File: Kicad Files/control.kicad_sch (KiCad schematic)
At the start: 77 parts, among them U35 74LS161, U36 SST39SF020, U37 SST39SF020, U38 SST39SF020, U39 SST39SF020

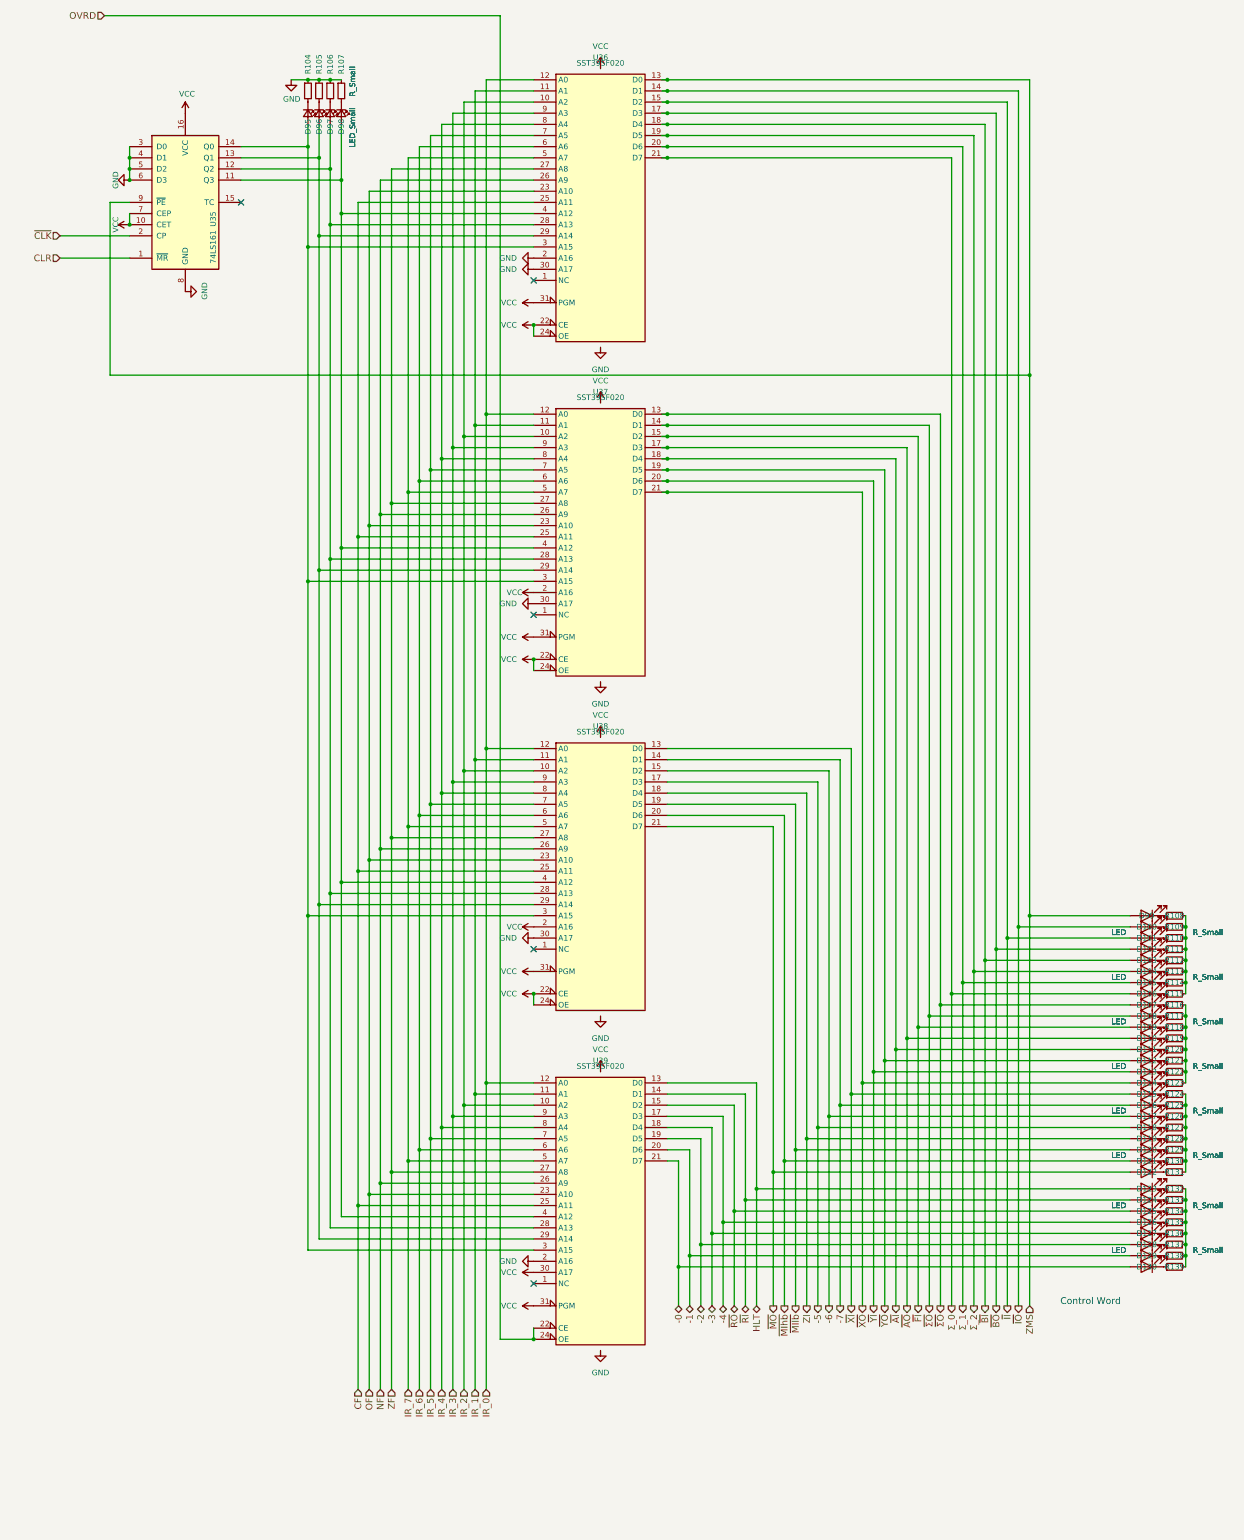
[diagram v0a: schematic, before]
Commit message: im sooo stupiiid
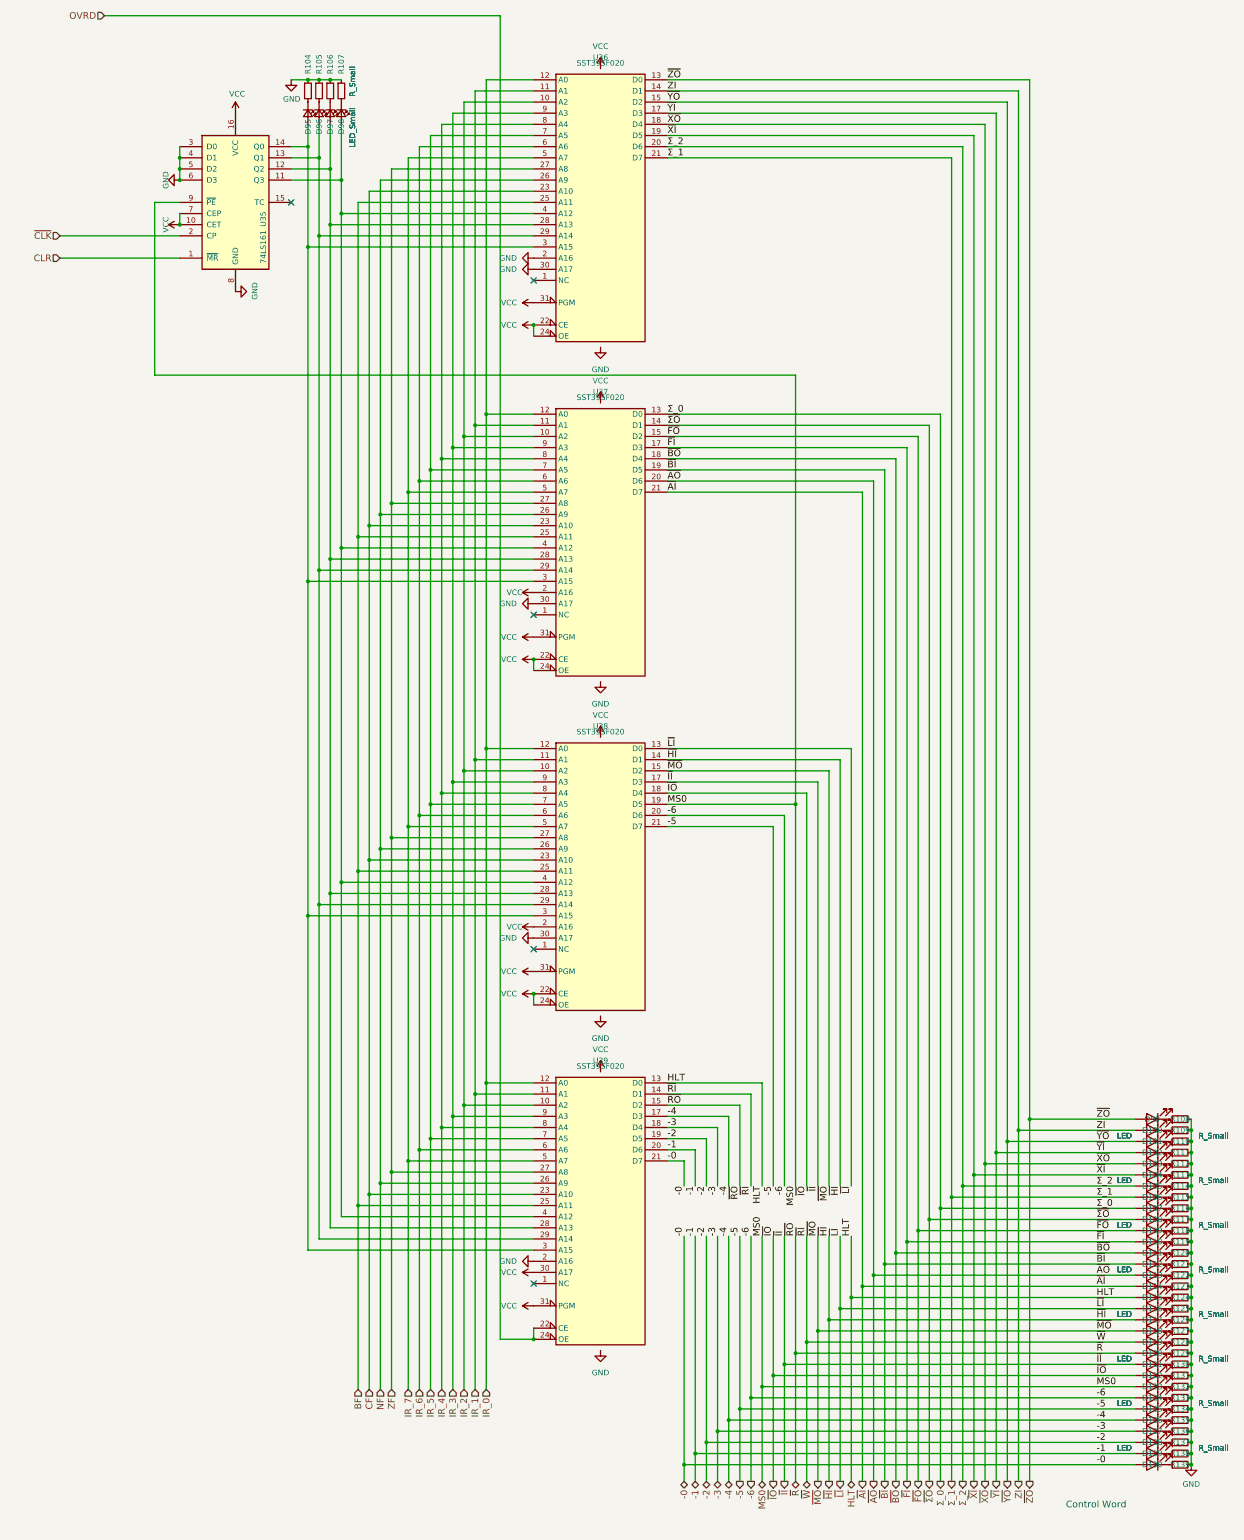
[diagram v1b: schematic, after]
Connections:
- net OF is gone; now on net CF: U36.23 (A10), U37.23 (A10), U38.23 (A10), U39.23 (A10)
- net -5: now also D125.2 (A), U38.21 (D7); no longer D118.2 (A), U38.17 (D3)
- net -6: now also D124.2 (A), U38.20 (D6); no longer D117.2 (A), U38.15 (D2)
- net CF: no longer U36.25 (A11), U37.25 (A11), U38.25 (A11), U39.25 (A11)
- net GND: now also R108.2, R109.2, R110.2, R111.2, R112.2, R113.2, R114.2, R115.2, R116.2, R117.2, R118.2, R119.2, R120.2, R121.2, R122.2, R123.2, R124.2, R125.2, R126.2, R127.2, R128.2, R129.2, R130.2, R131.2, R132.2, R133.2, R134.2, R135.2, R136.2, R137.2, R138.2, R139.2
- net HLT: now also D115.2 (A); no longer D123.2 (A)
- net ZI: now also D100.2 (A), U36.14 (D1); no longer D119.2 (A), U38.18 (D4)
- net ~{AI}: now also D114.2 (A), U37.21 (D7); no longer D111.2 (A), U37.18 (D4)
- net ~{AO}: now also D113.2 (A), U37.20 (D6); no longer D110.2 (A), U37.17 (D3)
- net ~{BI}: now also D112.2 (A), U37.19 (D5); no longer D103.2 (A), U36.18 (D4)
- net ~{BO}: now also D111.2 (A), U37.18 (D4); no longer D102.2 (A), U36.17 (D3)
- net ~{FI}: now also D110.2 (A), U37.17 (D3); no longer D109.2 (A), U37.15 (D2)
- net ~{II}: now also D121.2 (A), U38.17 (D3); no longer D101.2 (A), U36.15 (D2)
- net ~{IO}: now also D122.2 (A), U38.18 (D4); no longer D100.2 (A), U36.14 (D1)
- net ~{MO}: now also D118.2 (A), U38.15 (D2); no longer D122.2 (A), U38.21 (D7)
- net ~{XI}: now also D104.2 (A), U36.19 (D5); no longer D115.2 (A), U38.13 (D0)
- net ~{XO}: now also D103.2 (A), U36.18 (D4); no longer D114.2 (A), U37.21 (D7)
- net ~{YI}: now also D102.2 (A), U36.17 (D3); no longer D113.2 (A), U37.20 (D6)
- net ~{YO}: now also D101.2 (A), U36.15 (D2); no longer D112.2 (A), U37.19 (D5)
- net ~{ΣO}: no longer D107.2 (A), U37.13 (D0)
- net Σ_0: now also D107.2 (A), U37.13 (D0); no longer D106.2 (A), U36.21 (D7)
- net Σ_1: now also D106.2 (A), U36.21 (D7); no longer D105.2 (A), U36.20 (D6)
- net Σ_2: now also D105.2 (A), U36.20 (D6); no longer D104.2 (A), U36.19 (D5)
- net -7 renamed ~{HI}
- net ~{HI}: now also D117.2 (A); no longer D116.2 (A)
- net ZMS renamed ~{ZO}
- net ~{ZO}: no longer U35.9 (~{PE})
- removed net ~{MIhb}: D121.2 (A), U38.20 (D6)
- net ~{MIlb} renamed MS0
- net MS0: now also D123.2 (A), U35.9 (~{PE}); no longer D120.2 (A)
- net ~{RI} renamed ~{W}
- net ~{W}: now also D119.2 (A); no longer D124.2 (A)
- net ~{RO} renamed ~{R}
- net ~{R}: now also D120.2 (A); no longer D125.2 (A)
- new net BF: U36.25 (A11), U37.25 (A11), U38.25 (A11), U39.25 (A11)
- new net ~{FO}: D109.2 (A), U37.15 (D2)
- new net ~{LI}: D116.2 (A), U38.13 (D0)
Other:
- moved on the sheet: D100, D101, D102, D103, D104, D105, D106, D107, D108, D109, D110, D111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
